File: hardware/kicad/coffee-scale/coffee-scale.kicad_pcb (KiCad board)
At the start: 2 copper layers, 82.5 x 43 mm, 56 parts, among them J1 Conn_01x08, J2 Conn_01x04, J3 Conn_01x02, J4 USB C, Q1 DMG3415U, Q2 S8550, Q3 BSS138, SW1 SW_Push, SW2 SW_Push, SW3 SW_Push, U1 ESP32-S3, U2 HX711, U3 MCP73832-5-OT, U4 AP2112/RT9080-3.3

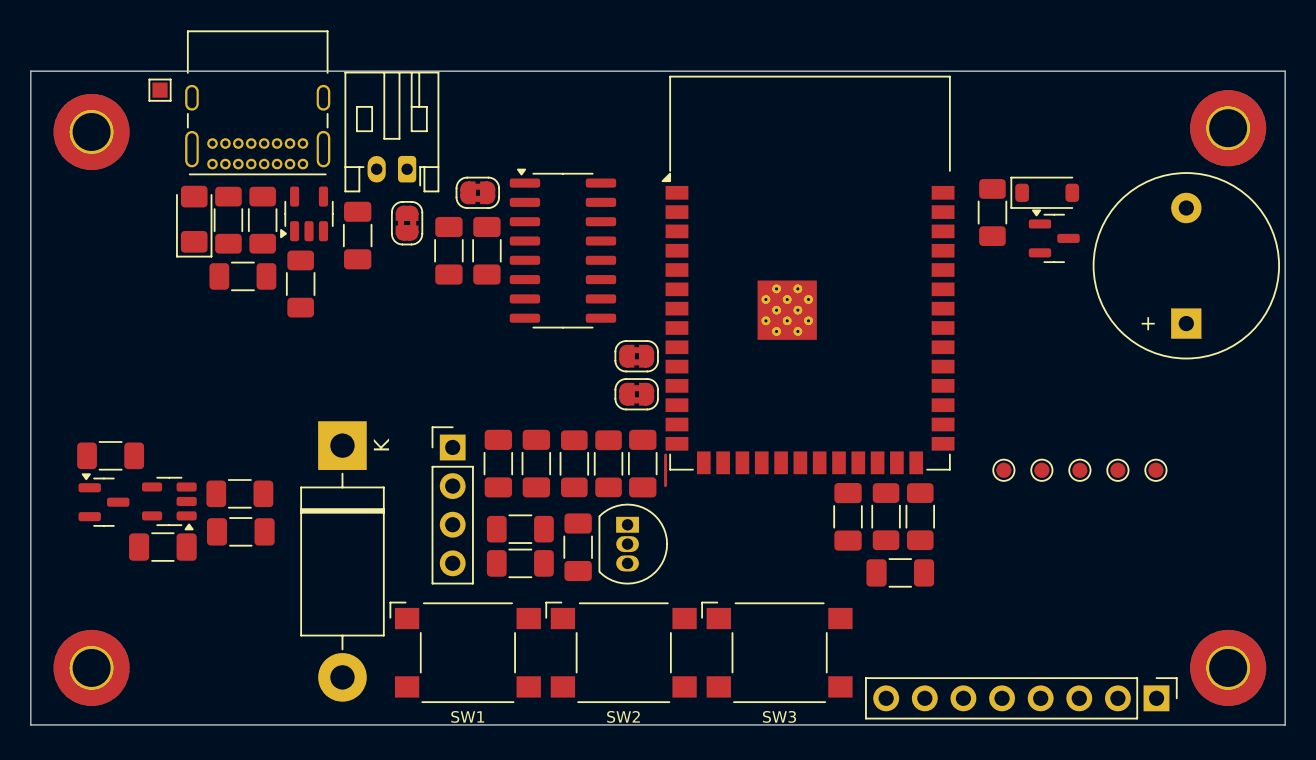
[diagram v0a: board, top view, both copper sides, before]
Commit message: update
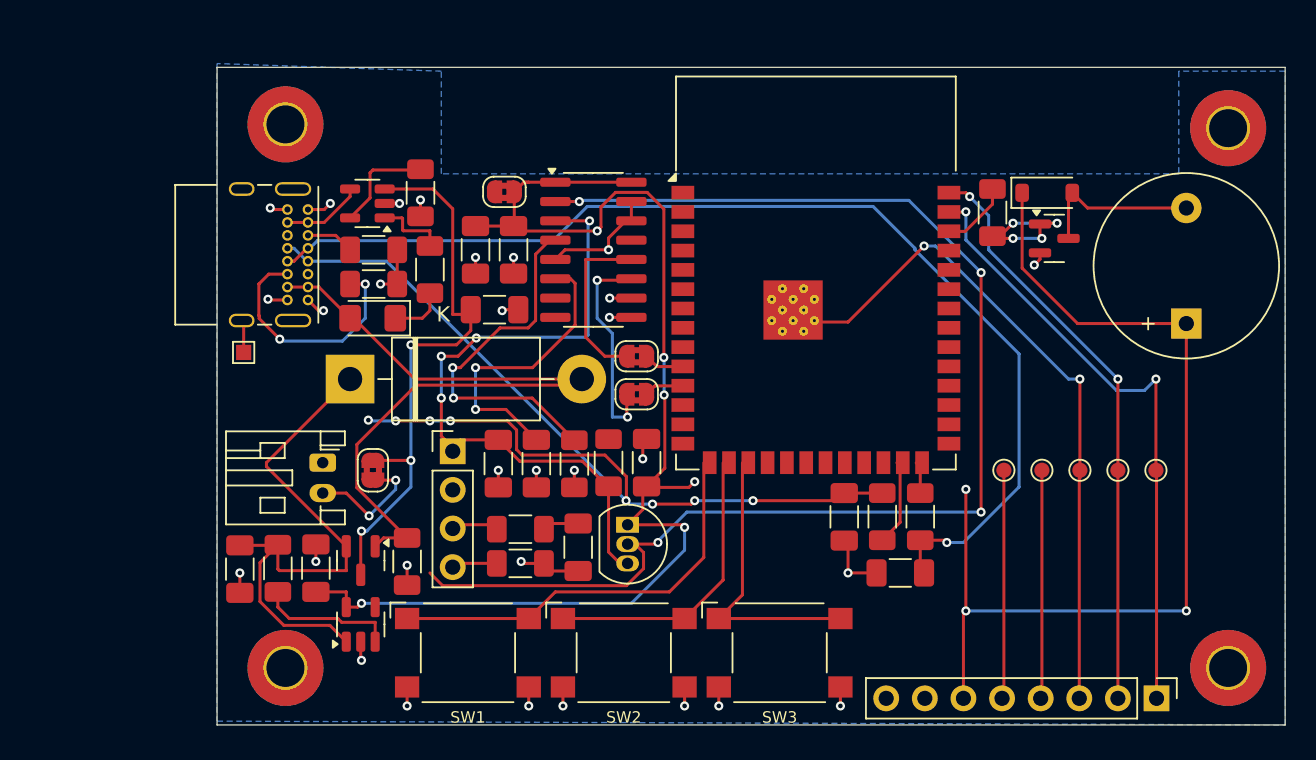
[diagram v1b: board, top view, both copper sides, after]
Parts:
- moved R2 20.7 mm to (141.5, 125.0), turned to -90 degrees
- moved J3 20.1 mm to (135.9, 118.5), turned to -90 degrees
- moved TP6 18.1 mm to (130.8, 111.2), turned to 90 degrees
- moved Q1 17.3 mm to (138.4, 124.9), turned to -90 degrees
- moved JP4 16.4 mm to (139.2, 119.0)
- moved U4 15.0 mm to (138.4, 129.1), turned to 90 degrees
- moved D2 13.4 mm to (139.2, 109.0), turned to 180 degrees
- moved H1 12.8 mm to (133.5, 96.2)
- moved H2 12.8 mm to (133.5, 132.0)
- moved R3 12.3 mm to (143.0, 105.8), turned to 90 degrees
- moved R9 10.4 mm to (139.3, 106.8), turned to 0 degrees
- moved C3 10.2 mm to (147.2, 108.4), turned to 0 degrees
- moved C2 10.2 mm to (135.5, 125.4), turned to 90 degrees
- moved R4 9.90 mm to (142.4, 100.8)
- moved R10 7.56 mm to (139.3, 104.5), turned to 0 degrees
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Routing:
- net 3.3V: track 0.00 -> 147.1 mm, vias 0 -> 9
- net Net-(Q2-B): track 0.00 -> 87.1 mm, vias 0 -> 4
- net /D+: track 0.00 -> 72.8 mm, vias 0 -> 1
- net /D-: track 0.00 -> 67.3 mm, vias 0 -> 8
- net VBUS: track 0.00 -> 55.1 mm
- net GND: track 0.14 -> 49.3 mm, vias 0 -> 29
- net /D/C: track 0.00 -> 44.6 mm, vias 0 -> 2
- net /E+: track 0.00 -> 43.9 mm, vias 0 -> 4
- net /CS: track 0.00 -> 41.3 mm, vias 0 -> 2
- net /RST: track 0.00 -> 38.9 mm, vias 0 -> 2
- net VBAT: track 0.00 -> 38.2 mm, vias 0 -> 3
- net Net-(D1-K): track 0.00 -> 36.7 mm
- net /BUT1: track 0.00 -> 27.4 mm
- net Net-(U2-VFB): track 2.00 -> 23.9 mm, vias 0 -> 2
- net Net-(U2-VBG): track 0.00 -> 19.5 mm, vias 0 -> 2
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- added copper zone on B.Cu, net GND
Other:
- board size 82.5 x 43 mm -> 70.2 x 43.2 mm
